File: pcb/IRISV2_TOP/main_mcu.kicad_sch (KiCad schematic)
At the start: 38 parts, among them IC1 ATA6561-GAQW-N, J10 Conn_02x04_Odd_Even, J4 Screw_Terminal_01x03, U4 STM32H563VITx, Y1 25mHz 8pf, Y2 32.768kHz 12.5pF

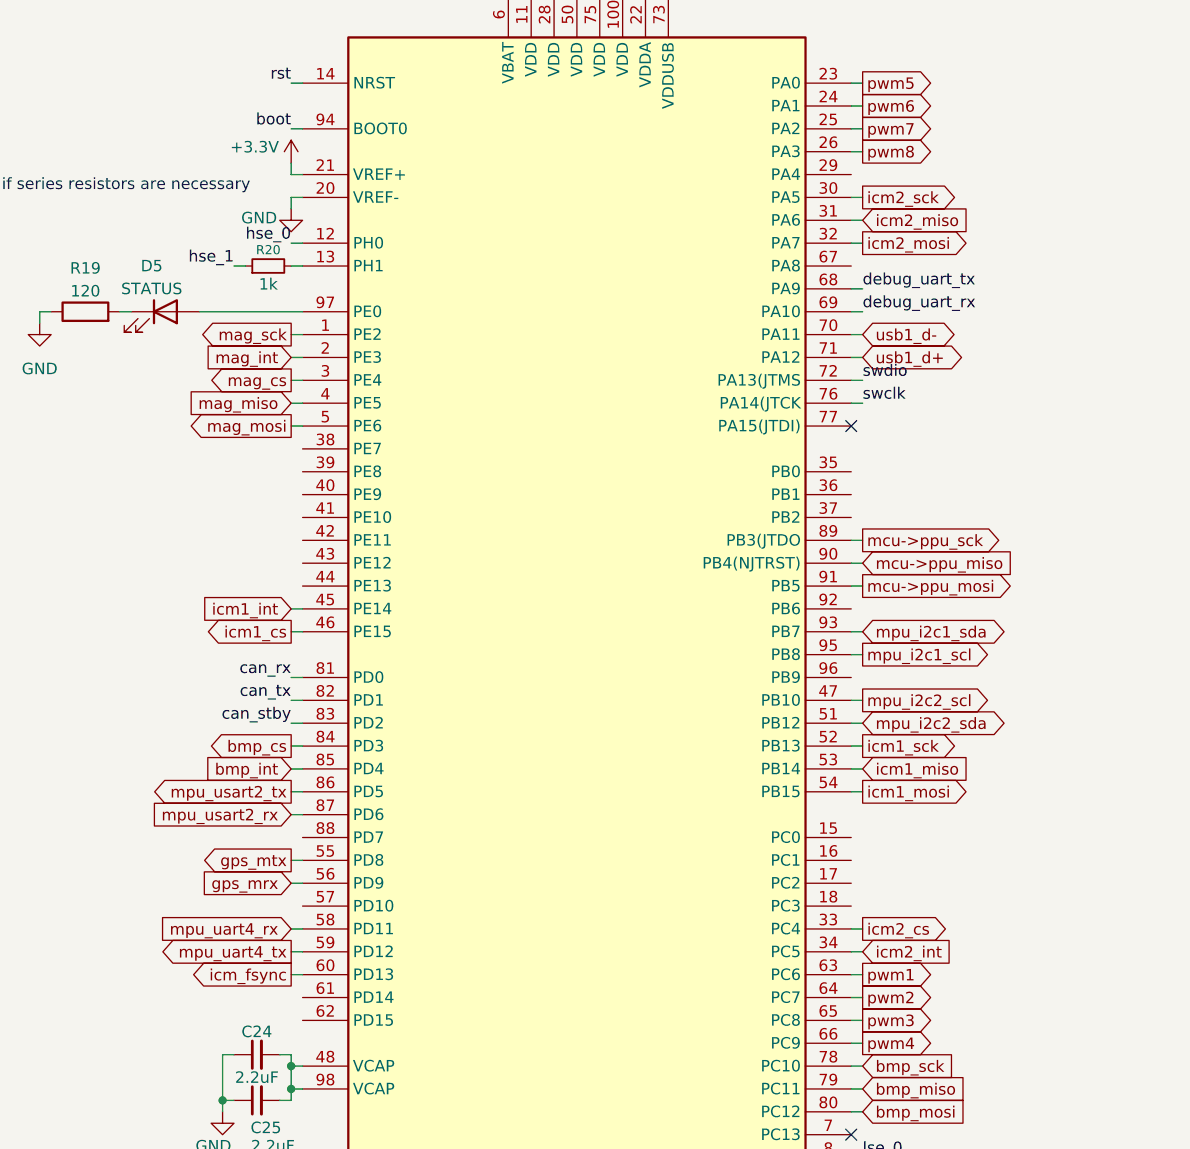
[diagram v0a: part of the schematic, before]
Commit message: most routing done inc some reassignment, pretty much just connectors left now
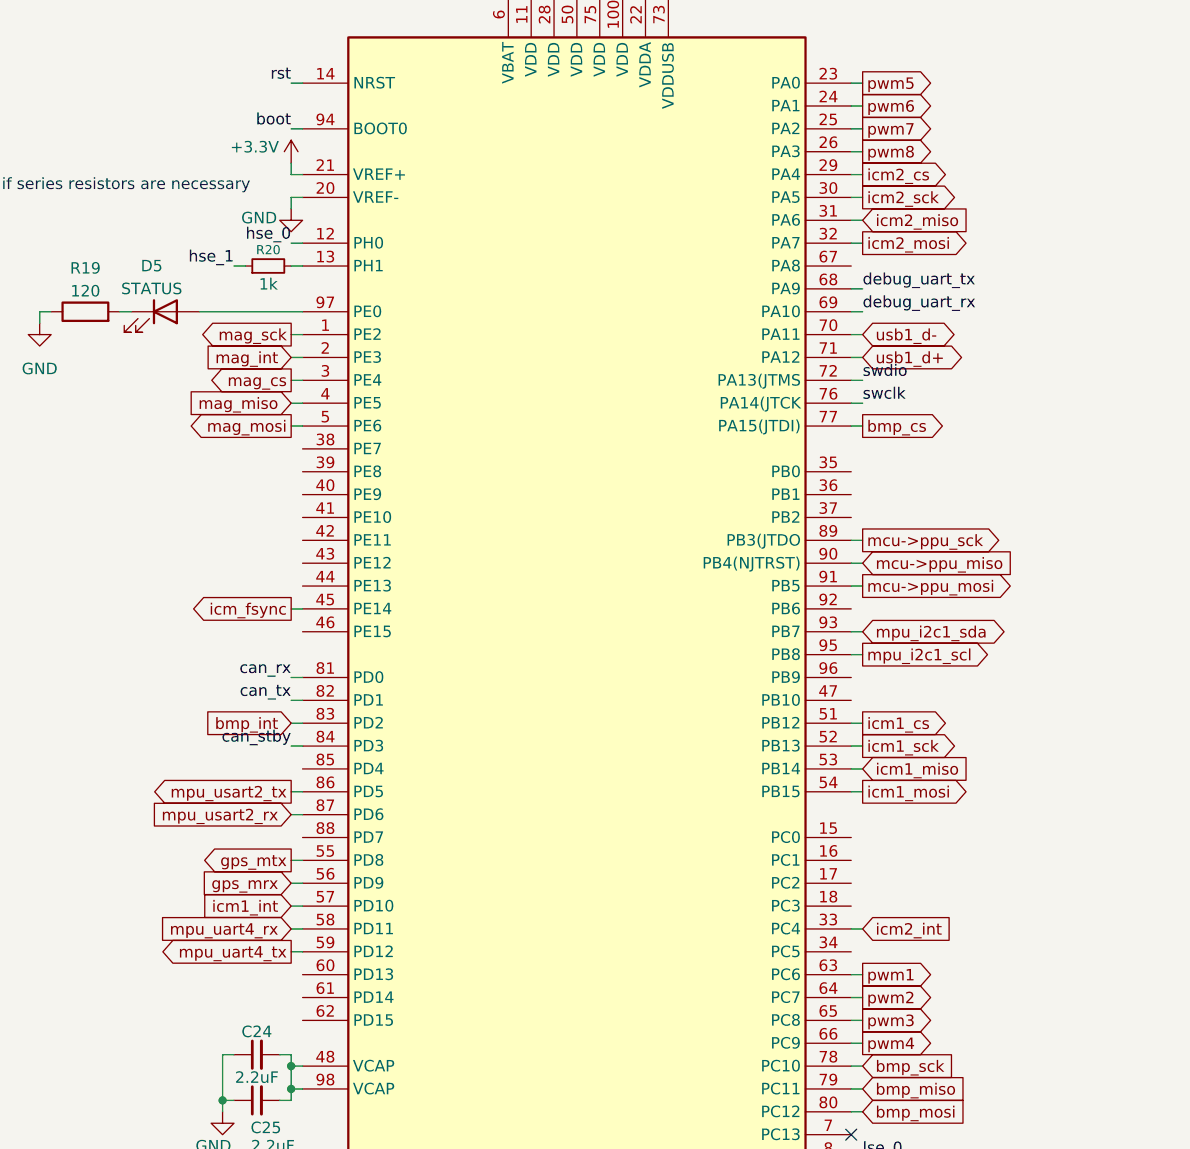
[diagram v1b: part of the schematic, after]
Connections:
- net mpu_i2c2_sda is gone; now on net icm1_cs: U4.51 (PB12)
- net bmp_cs: now also U4.77 (PA15(JTDI)); no longer U4.84 (PD3)
- net bmp_int: now also U4.83 (PD2); no longer U4.85 (PD4)
- net can_stby: now also U4.84 (PD3); no longer U4.83 (PD2)
- net icm1_cs: no longer U4.46 (PE15)
- net icm1_int: now also U4.57 (PD10); no longer U4.45 (PE14)
- net icm2_cs: now also U4.29 (PA4); no longer U4.33 (PC4)
- net icm2_int: now also U4.33 (PC4); no longer U4.34 (PC5)
- net icm_fsync: now also U4.45 (PE14); no longer U4.60 (PD13)
- net mpu_i2c2_scl: no longer names the net of U4.47 (PB10)
- no-connect marks 2 -> 1
